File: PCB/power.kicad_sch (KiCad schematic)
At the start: 22 parts, among them Q1 AO3401A, U1 LP2951-33DR, U2 AMS1117

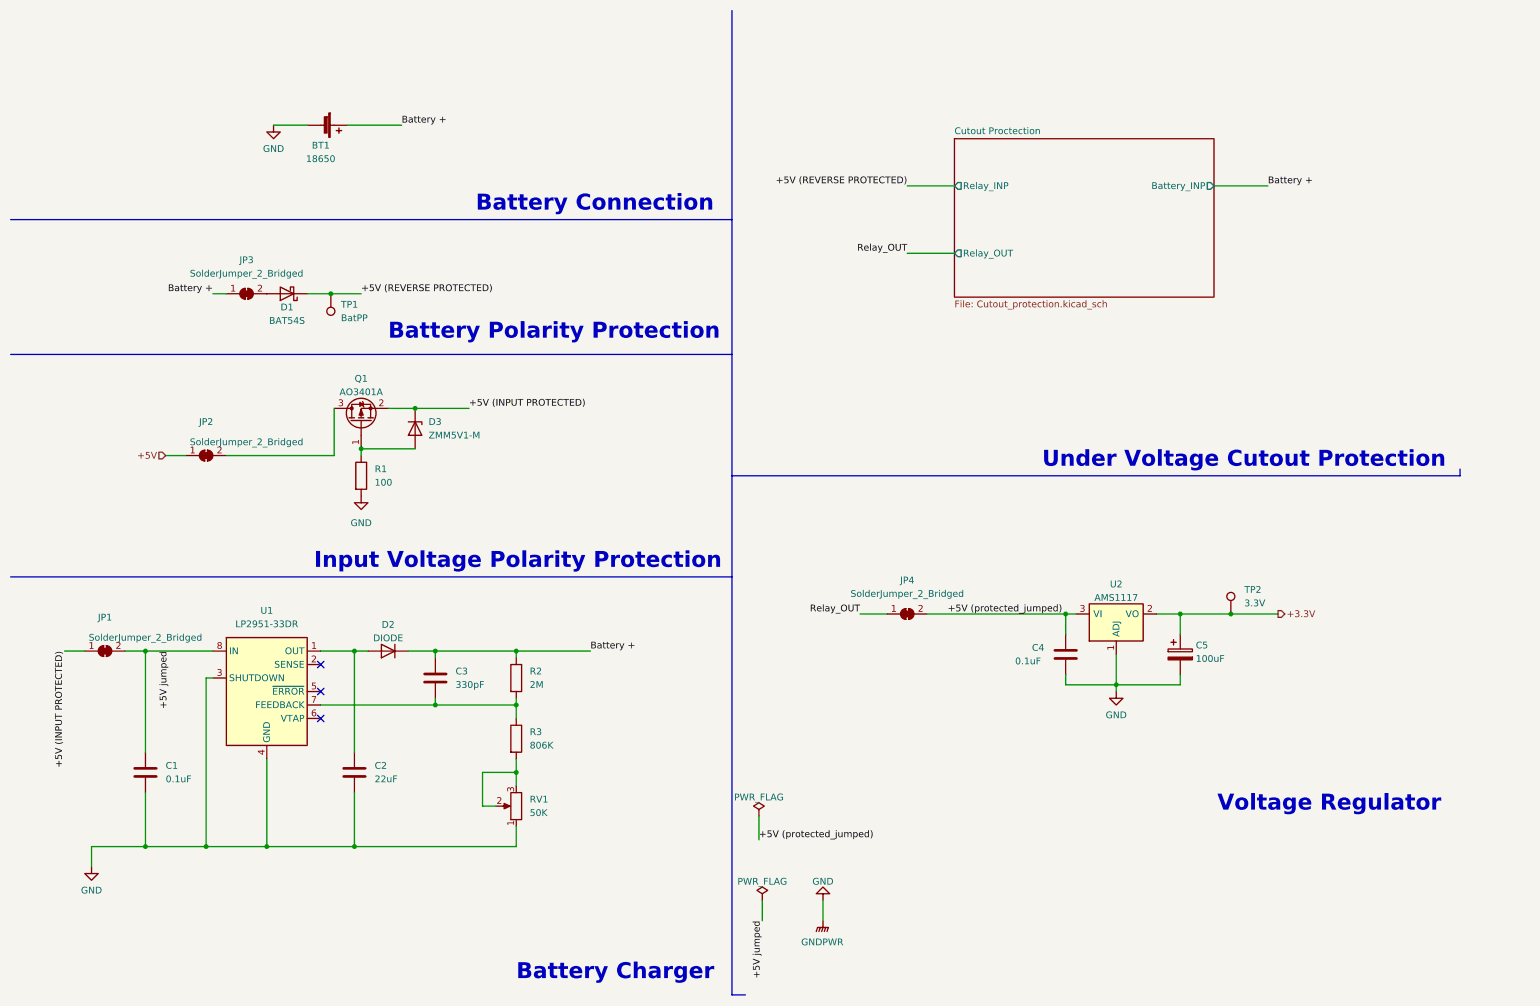
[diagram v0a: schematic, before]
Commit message: POWER CHANGES YAAASSSSSSS
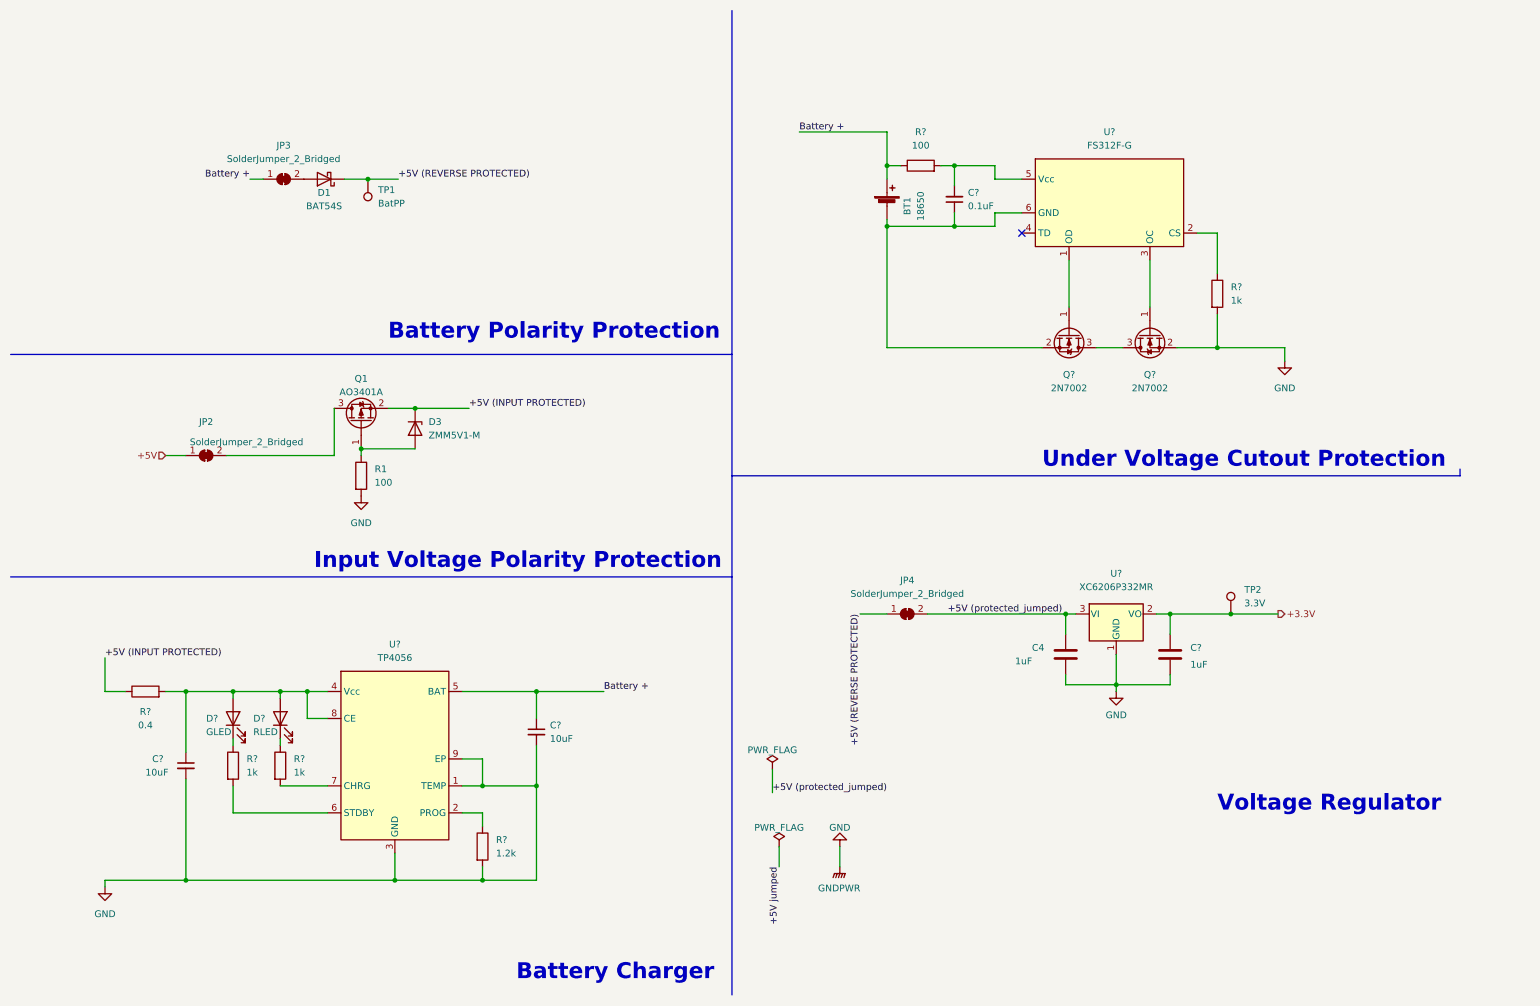
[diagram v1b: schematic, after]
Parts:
- removed C1: 0.1uF, Capacitor_SMD:C_0402_1005Metric, symbol Device:C
- removed C2: 22uF, Capacitor_SMD:C_0603_1608Metric, symbol Device:C
- removed C3: 330pF, Capacitor_SMD:C_0402_1005Metric, symbol Device:C
- removed C5: 100uF, Capacitor_SMD:C_1206_3216Metric, symbol Device:C_Polarized
- removed D2: DIODE, Footprint_EEE3088F:DO-214AC_L4.3-W2.7-LS5.3-RD, symbol Simulation_SPICE:DIODE
- removed JP1: SolderJumper_2_Bridged, Jumper:SolderJumper-2_P1.3mm_Bridged2Bar_Pad1.0x1.5mm, symbol Jumper:SolderJumper_2_Bridged
- removed R2: 2M, Resistor_SMD:R_0805_2012Metric, symbol Device:R
- removed R3: 806K, Resistor_SMD:R_0402_1005Metric, symbol Device:R
- removed RV1: 50K, Footprint_EEE3088F:VG039NCHXTB503, symbol Device:R_Potentiometer
- removed U1: LP2951-33DR, Package_SO:SOIC-8_3.9x4.9mm_P1.27mm, symbol Regulator_Linear:LP2951-3.3_DIP
- removed U2: AMS1117, Package_TO_SOT_SMD:SOT-223-3_TabPin2, symbol Regulator_Linear:AMS1117
- added C?: 1uF, Capacitor_SMD:C_0402_1005Metric, symbol Device:C
- added C?: 0.1uF, symbol Device:C_Small
- added C? (x2): 10uF, symbol Device:C_Small
- added D?: RLED, symbol Device:LED
- added D?: GLED, symbol Device:LED
- added Q? (x2): 2N7002, Package_TO_SOT_SMD:SOT-23, symbol Transistor_FET:2N7002
- added R?: 100, symbol Device:R
- added R? (x3): 1k, symbol Device:R
- added R?: 1.2k, symbol Device:R
- added R?: 0.4, symbol Device:R
- added U?: FS312F-G, symbol Battery_Management:FS312F-G
- added U?: TP4056, symbol Battery_Management:TP4056
- added U?: XC6206P332MR, Package_TO_SOT_SMD:SOT-23, symbol Regulator_Linear:XC6206PxxxMR
- C4: value 0.1uF -> 1uF
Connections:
- net Relay_OUT is gone; now on net +5V (REVERSE PROTECTED): JP4.1 (A)
- net +3.3V: now also C?.1, U?.2 (VO)
- net +5V (INPUT PROTECTED): now also R?.1
- net +5V (protected_jumped): now also U?.3 (VI)
- net Battery +: now also C?.1, R?.1, U?.5 (BAT)
- net GND: now also C?.2, C?.2, C?.2, Q?.2 (S), R?.2, R?.2, U?.1 (GND), U?.1 (TEMP), U?.3 (GND), U?.9 (EP); no longer BT1.2 (-)
- new net: BT1.2 (-), C?.1, Q?.2 (S), U?.6 (GND)
- new net: C?.2, R?.2, U?.5 (Vcc)
- new net: Q?.1 (G), U?.1 (OD)
- new net: R?.1, U?.2 (CS)
- new net: Q?.1 (G), U?.3 (OC)
- new net: D?.1 (K), R?.1 (x2)
- new net: C?.1, D?.2 (A), D?.2 (A), R?.2, U?.4 (Vcc), U?.8 (CE)
- new net: R?.1, U?.2 (PROG)
- new net: R?.2, U?.6 (STDBY)
- new net: R?.2, U?.7 (CHRG)
- new net: Q?.3 (D), Q?.3 (D)
- no-connect marks 3 -> 1
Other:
- removed sheet Cutout Proctection
- note removed: "Battery Connection"
- moved on the sheet: BT1, D1, JP3, TP1
